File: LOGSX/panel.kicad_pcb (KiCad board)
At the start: 4 copper layers, 84 x 98 mm, 18 parts

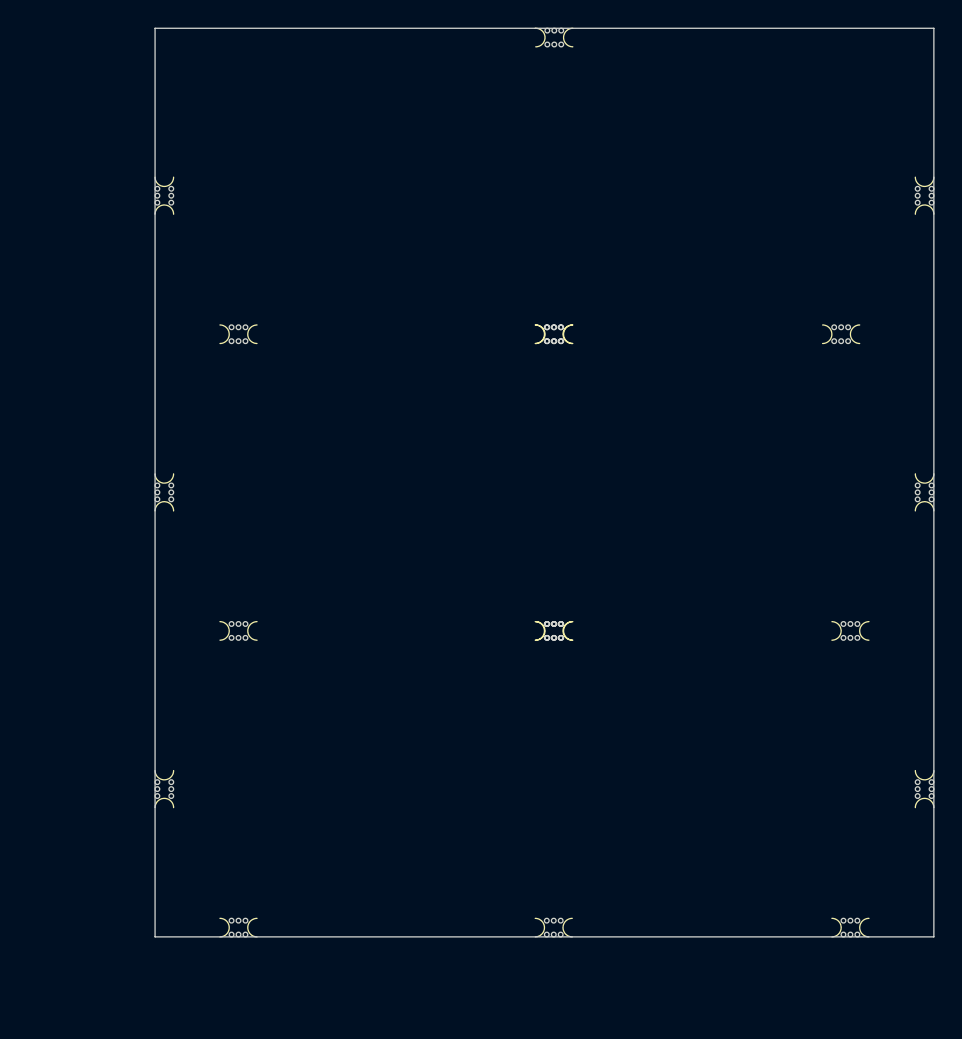
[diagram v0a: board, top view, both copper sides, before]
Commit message: Add files via upload
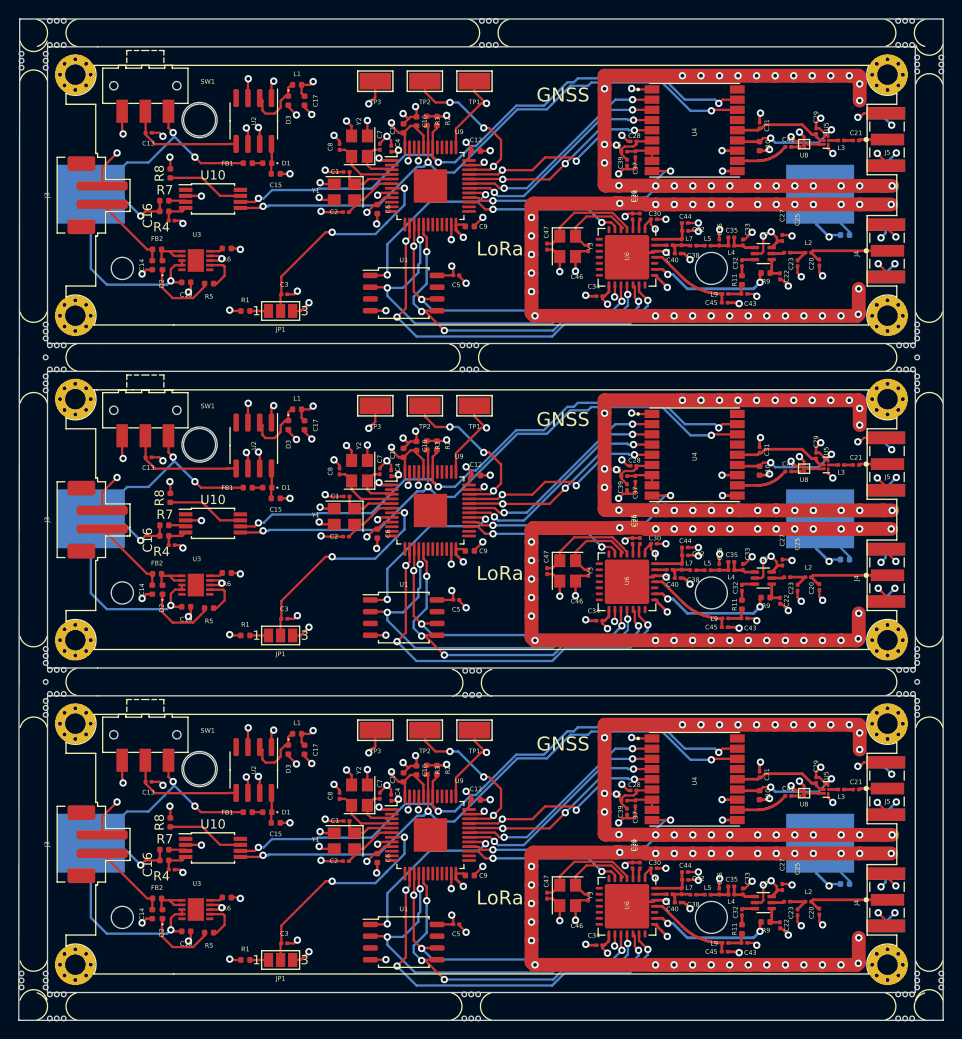
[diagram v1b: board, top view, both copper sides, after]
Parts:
- removed mouse-bite-2mm-slot (x18): VAL**, ASSETS:mouse-bite-2mm-slot
- added C1: 2.2pF, Capacitor_SMD:C_0201_0603Metric, F.Cu at (162.7, 138.5)
- added C1: 2.2pF, Capacitor_SMD:C_0201_0603Metric, F.Cu at (162.7, 103.5)
- added C1: 2.2pF, Capacitor_SMD:C_0201_0603Metric, F.Cu at (162.7, 68.5)
- added C10: 2.2pF, Capacitor_SMD:C_0402_1005Metric, F.Cu at (170.2, 133.0)
- added C10: 2.2pF, Capacitor_SMD:C_0402_1005Metric, F.Cu at (170.2, 98.0)
- added C10: 2.2pF, Capacitor_SMD:C_0402_1005Metric, F.Cu at (170.2, 63.0)
- added C11: 2.2pF, Capacitor_SMD:C_0402_1005Metric, F.Cu at (168.8, 133.8)
- added C11: 2.2pF, Capacitor_SMD:C_0402_1005Metric, F.Cu at (168.8, 98.8)
- added C11: 2.2pF, Capacitor_SMD:C_0402_1005Metric, F.Cu at (168.8, 63.8)
- added C12: 2.2pF, Capacitor_SMD:C_0402_1005Metric, F.Cu at (176.6, 136.2)
- added C12: 2.2pF, Capacitor_SMD:C_0402_1005Metric, F.Cu at (176.6, 101.2)
- added C12: 2.2pF, Capacitor_SMD:C_0402_1005Metric, F.Cu at (176.6, 66.2)
- added C13: 1nF, Capacitor_SMD:C_0201_0603Metric, F.Cu at (141.3, 134.3)
- added C13: 1nF, Capacitor_SMD:C_0201_0603Metric, F.Cu at (141.3, 99.3)
- added C13: 1nF, Capacitor_SMD:C_0201_0603Metric, F.Cu at (141.3, 64.3)
- added C14: 22pF, Capacitor_SMD:C_0402_1005Metric, F.Cu at (141.7, 148.6)
- added C14: 22pF, Capacitor_SMD:C_0402_1005Metric, F.Cu at (141.7, 113.5)
- added C14: 22pF, Capacitor_SMD:C_0402_1005Metric, F.Cu at (141.7, 78.5)
- added C15: 1uF, Capacitor_SMD:C_0402_1005Metric, F.Cu at (155.0, 138.7)
- added C15: 1uF, Capacitor_SMD:C_0402_1005Metric, F.Cu at (155.0, 103.7)
- added C15: 1uF, Capacitor_SMD:C_0402_1005Metric, F.Cu at (155.0, 68.7)
- added C16: 1nF, Capacitor_SMD:C_0201_0603Metric, F.Cu at (143.8, 143.8)
- added C16: 1nF, Capacitor_SMD:C_0201_0603Metric, F.Cu at (143.8, 108.8)
- added C16: 1nF, Capacitor_SMD:C_0201_0603Metric, F.Cu at (143.8, 73.8)
- added C17: 330uF, Capacitor_SMD:C_0402_1005Metric, F.Cu at (158.1, 130.8)
- added C17: 330uF, Capacitor_SMD:C_0402_1005Metric, F.Cu at (158.1, 95.8)
- added C17: 330uF, Capacitor_SMD:C_0402_1005Metric, F.Cu at (158.1, 60.8)
- added C19: 22pF, Capacitor_SMD:C_0402_1005Metric, F.Cu at (145.4, 150.4)
- added C19: 22pF, Capacitor_SMD:C_0402_1005Metric, F.Cu at (145.4, 115.4)
- added C19: 22pF, Capacitor_SMD:C_0402_1005Metric, F.Cu at (145.4, 80.4)
- added C2: 2.2pF, Capacitor_SMD:C_0201_0603Metric, F.Cu at (162.6, 142.8)
- added C2: 2.2pF, Capacitor_SMD:C_0201_0603Metric, F.Cu at (162.6, 107.8)
- added C2: 2.2pF, Capacitor_SMD:C_0201_0603Metric, F.Cu at (162.6, 72.8)
- added C20: X, Capacitor_SMD:C_0201_0603Metric, F.Cu at (213.7, 148.3)
- added C20: X, Capacitor_SMD:C_0201_0603Metric, F.Cu at (213.7, 113.3)
- added C20: X, Capacitor_SMD:C_0201_0603Metric, F.Cu at (213.7, 78.3)
- added C21: 120pF, Capacitor_SMD:C_0201_0603Metric, F.Cu at (217.6, 135.1)
- added C21: 120pF, Capacitor_SMD:C_0201_0603Metric, F.Cu at (217.6, 100.1)
- added C21: 120pF, Capacitor_SMD:C_0201_0603Metric, F.Cu at (217.6, 65.1)
- added C22: 1nF, Capacitor_SMD:C_0201_0603Metric, F.Cu at (209.4, 149.8)
- added C22: 1nF, Capacitor_SMD:C_0201_0603Metric, F.Cu at (209.4, 114.8)
- added C22: 1nF, Capacitor_SMD:C_0201_0603Metric, F.Cu at (209.4, 79.8)
- added C23: X, Capacitor_SMD:C_0201_0603Metric, F.Cu at (211.3, 148.3)
- added C23: X, Capacitor_SMD:C_0201_0603Metric, F.Cu at (211.3, 113.3)
- added C23: X, Capacitor_SMD:C_0201_0603Metric, F.Cu at (211.3, 78.3)
- added C24: 100nF, Capacitor_SMD:C_0201_0603Metric, F.Cu at (194.3, 143.3)
- added C24: 100nF, Capacitor_SMD:C_0201_0603Metric, F.Cu at (194.3, 108.3)
- added C24: 100nF, Capacitor_SMD:C_0201_0603Metric, F.Cu at (194.3, 73.3)
- added C25: X, Capacitor_SMD:C_0201_0603Metric, F.Cu at (210.2, 147.2)
- added C25: X, Capacitor_SMD:C_0201_0603Metric, F.Cu at (210.2, 112.2)
- added C25: X, Capacitor_SMD:C_0201_0603Metric, F.Cu at (210.2, 77.2)
- added C26: 100nF, Capacitor_SMD:C_0201_0603Metric, F.Cu at (193.5, 143.3)
- added C26: 100nF, Capacitor_SMD:C_0201_0603Metric, F.Cu at (193.5, 108.3)
- added C26: 100nF, Capacitor_SMD:C_0201_0603Metric, F.Cu at (193.5, 73.3)
- added C27: 1nF, Capacitor_SMD:C_0201_0603Metric, F.Cu at (209.7, 145.6)
- added C27: 1nF, Capacitor_SMD:C_0201_0603Metric, F.Cu at (209.7, 110.6)
- added C27: 1nF, Capacitor_SMD:C_0201_0603Metric, F.Cu at (209.7, 75.6)
- added C28: 56pF, Capacitor_SMD:C_0201_0603Metric, F.Cu at (193.6, 135.2)
- added C28: 56pF, Capacitor_SMD:C_0201_0603Metric, F.Cu at (193.6, 100.2)
- added C28: 56pF, Capacitor_SMD:C_0201_0603Metric, F.Cu at (193.6, 65.2)
- added C29: 1nF, Capacitor_SMD:C_0201_0603Metric, F.Cu at (213.3, 134.1)
- added C29: 1nF, Capacitor_SMD:C_0201_0603Metric, F.Cu at (213.3, 99.1)
- added C29: 1nF, Capacitor_SMD:C_0201_0603Metric, F.Cu at (213.3, 64.1)
- added C3: 2.2pF, Capacitor_SMD:C_0201_0603Metric, F.Cu at (155.9, 151.7)
- added C3: 2.2pF, Capacitor_SMD:C_0201_0603Metric, F.Cu at (155.9, 116.7)
- added C3: 2.2pF, Capacitor_SMD:C_0201_0603Metric, F.Cu at (155.9, 81.7)
- added C30: 100nF, Capacitor_SMD:C_0201_0603Metric, F.Cu at (195.8, 143.6)
- added C30: 100nF, Capacitor_SMD:C_0201_0603Metric, F.Cu at (195.8, 108.6)
- added C30: 100nF, Capacitor_SMD:C_0201_0603Metric, F.Cu at (195.8, 73.6)
- added C31: 56pF, Capacitor_SMD:C_0201_0603Metric, F.Cu at (207.2, 133.5)
- added C31: 56pF, Capacitor_SMD:C_0201_0603Metric, F.Cu at (207.2, 98.5)
- added C31: 56pF, Capacitor_SMD:C_0201_0603Metric, F.Cu at (207.2, 63.5)
- added C32: 120pF, Capacitor_SMD:C_0201_0603Metric, F.Cu at (205.3, 148.3)
- added C32: 120pF, Capacitor_SMD:C_0201_0603Metric, F.Cu at (205.3, 113.3)
- added C32: 120pF, Capacitor_SMD:C_0201_0603Metric, F.Cu at (205.3, 78.3)
- added C33: X, Capacitor_SMD:C_0201_0603Metric, F.Cu at (205.4, 146.1)
- added C33: X, Capacitor_SMD:C_0201_0603Metric, F.Cu at (205.4, 111.1)
- added C33: X, Capacitor_SMD:C_0201_0603Metric, F.Cu at (205.4, 76.1)
- added C34: 100nF, Capacitor_SMD:C_0201_0603Metric, F.Cu at (189.9, 151.9)
- added C34: 100nF, Capacitor_SMD:C_0201_0603Metric, F.Cu at (189.9, 116.9)
- added C34: 100nF, Capacitor_SMD:C_0201_0603Metric, F.Cu at (189.9, 81.9)
- added C35: X, Capacitor_SMD:C_0201_0603Metric, F.Cu at (204.2, 145.6)
- added C35: X, Capacitor_SMD:C_0201_0603Metric, F.Cu at (204.2, 110.5)
- added C35: X, Capacitor_SMD:C_0201_0603Metric, F.Cu at (204.2, 75.5)
- added C36: X, Capacitor_SMD:C_0201_0603Metric, F.Cu at (202.8, 146.1)
- added C36: X, Capacitor_SMD:C_0201_0603Metric, F.Cu at (202.8, 111.1)
- added C36: X, Capacitor_SMD:C_0201_0603Metric, F.Cu at (202.8, 76.1)
- added C37: 56pF, Capacitor_SMD:C_0201_0603Metric, F.Cu at (193.8, 136.6)
- added C37: 56pF, Capacitor_SMD:C_0201_0603Metric, F.Cu at (193.8, 101.6)
- added C37: 56pF, Capacitor_SMD:C_0201_0603Metric, F.Cu at (193.8, 66.6)
- added C38: X, Capacitor_SMD:C_0201_0603Metric, F.Cu at (200.1, 146.4)
- added C38: X, Capacitor_SMD:C_0201_0603Metric, F.Cu at (200.1, 111.5)
- added C38: X, Capacitor_SMD:C_0201_0603Metric, F.Cu at (200.1, 76.5)
- added C39: 56pF, Capacitor_SMD:C_0201_0603Metric, F.Cu at (192.9, 137.5)
- added C39: 56pF, Capacitor_SMD:C_0201_0603Metric, F.Cu at (192.9, 102.5)
- added C39: 56pF, Capacitor_SMD:C_0201_0603Metric, F.Cu at (192.9, 67.5)
- added C4: 2.2pF, Capacitor_SMD:C_0201_0603Metric, F.Cu at (167.5, 136.0)
- added C4: 2.2pF, Capacitor_SMD:C_0201_0603Metric, F.Cu at (167.5, 101.0)
- added C4: 2.2pF, Capacitor_SMD:C_0201_0603Metric, F.Cu at (167.5, 66.0)
- added C40: X, Capacitor_SMD:C_0201_0603Metric, F.Cu at (198.4, 147.3)
- added C40: X, Capacitor_SMD:C_0201_0603Metric, F.Cu at (198.4, 112.3)
- added C40: X, Capacitor_SMD:C_0201_0603Metric, F.Cu at (198.4, 77.3)
- added C41: 120pF, Capacitor_SMD:C_0201_0603Metric, F.Cu at (210.3, 135.8)
- added C41: 120pF, Capacitor_SMD:C_0201_0603Metric, F.Cu at (210.3, 100.8)
- added C41: 120pF, Capacitor_SMD:C_0201_0603Metric, F.Cu at (210.3, 65.8)
- added C42: X, Capacitor_SMD:C_0201_0603Metric, F.Cu at (199.2, 144.8)
- added C42: X, Capacitor_SMD:C_0201_0603Metric, F.Cu at (199.2, 109.8)
- added C42: X, Capacitor_SMD:C_0201_0603Metric, F.Cu at (199.2, 74.8)
- added C43: X, Capacitor_SMD:C_0201_0603Metric, F.Cu at (205.6, 151.7)
- added C43: X, Capacitor_SMD:C_0201_0603Metric, F.Cu at (205.6, 116.7)
- added C43: X, Capacitor_SMD:C_0201_0603Metric, F.Cu at (205.6, 81.7)
- added C44: X, Capacitor_SMD:C_0201_0603Metric, F.Cu at (199.2, 144.0)
- added C44: X, Capacitor_SMD:C_0201_0603Metric, F.Cu at (199.2, 109.0)
- added C44: X, Capacitor_SMD:C_0201_0603Metric, F.Cu at (199.2, 74.0)
- added C45: X, Capacitor_SMD:C_0201_0603Metric, F.Cu at (203.4, 152.6)
- added C45: X, Capacitor_SMD:C_0201_0603Metric, F.Cu at (203.4, 117.6)
- added C45: X, Capacitor_SMD:C_0201_0603Metric, F.Cu at (203.4, 82.6)
- added C46: 2.2pF, Capacitor_SMD:C_0201_0603Metric, F.Cu at (188.7, 146.7)
- added C46: 2.2pF, Capacitor_SMD:C_0201_0603Metric, F.Cu at (188.7, 111.7)
- added C46: 2.2pF, Capacitor_SMD:C_0201_0603Metric, F.Cu at (188.7, 76.7)
- added C47: 2.2pF, Capacitor_SMD:C_0201_0603Metric, F.Cu at (184.3, 146.6)
- added C47: 2.2pF, Capacitor_SMD:C_0201_0603Metric, F.Cu at (184.3, 111.5)
- added C47: 2.2pF, Capacitor_SMD:C_0201_0603Metric, F.Cu at (184.3, 76.5)
- added C5: 2.2pF, Capacitor_SMD:C_0201_0603Metric, F.Cu at (174.5, 149.6)
- added C5: 2.2pF, Capacitor_SMD:C_0201_0603Metric, F.Cu at (174.5, 114.6)
- added C5: 2.2pF, Capacitor_SMD:C_0201_0603Metric, F.Cu at (174.5, 79.6)
- added C6: 1uF, Capacitor_SMD:C_0402_1005Metric, F.Cu at (166.0, 142.5)
- added C6: 1uF, Capacitor_SMD:C_0402_1005Metric, F.Cu at (166.0, 107.5)
- added C6: 1uF, Capacitor_SMD:C_0402_1005Metric, F.Cu at (166.0, 72.5)
- added C7: 1pF, Capacitor_SMD:C_0201_0603Metric, F.Cu at (166.2, 135.8)
- added C7: 1pF, Capacitor_SMD:C_0201_0603Metric, F.Cu at (166.2, 100.8)
- added C7: 1pF, Capacitor_SMD:C_0201_0603Metric, F.Cu at (166.2, 65.8)
- added C8: 1pF, Capacitor_SMD:C_0201_0603Metric, F.Cu at (161.9, 135.8)
- added C8: 1pF, Capacitor_SMD:C_0201_0603Metric, F.Cu at (161.9, 100.8)
- added C8: 1pF, Capacitor_SMD:C_0201_0603Metric, F.Cu at (161.9, 65.8)
- added C9: 2.2pF, Capacitor_SMD:C_0402_1005Metric, F.Cu at (175.9, 144.4)
- added C9: 2.2pF, Capacitor_SMD:C_0402_1005Metric, F.Cu at (175.9, 109.4)
- added C9: 2.2pF, Capacitor_SMD:C_0402_1005Metric, F.Cu at (175.9, 74.4)
- added D1: D_Small, Diode_SMD:D_0402_1005Metric, F.Cu at (154.1, 137.6)
- added D1: D_Small, Diode_SMD:D_0402_1005Metric, F.Cu at (154.1, 102.5)
- added D1: D_Small, Diode_SMD:D_0402_1005Metric, F.Cu at (154.1, 67.5)
- added D2: LED, LED_SMD:LED_0402_1005Metric, F.Cu at (142.8, 148.6)
- added D2: LED, LED_SMD:LED_0402_1005Metric, F.Cu at (142.8, 113.5)
- added D2: LED, LED_SMD:LED_0402_1005Metric, F.Cu at (142.8, 78.5)
- added D3: 1N5822, Diode_SMD:D_0402_1005Metric, F.Cu at (156.4, 130.8)
- added D3: 1N5822, Diode_SMD:D_0402_1005Metric, F.Cu at (156.4, 95.8)
- added D3: 1N5822, Diode_SMD:D_0402_1005Metric, F.Cu at (156.4, 60.8)
- added FB1: 100MHz, Inductor_SMD:L_0402_1005Metric, F.Cu at (152.0, 137.6)
- added FB1: 100MHz, Inductor_SMD:L_0402_1005Metric, F.Cu at (152.0, 102.5)
- added FB1: 100MHz, Inductor_SMD:L_0402_1005Metric, F.Cu at (152.0, 67.5)
- added FB2: 100MHz, Inductor_SMD:L_0402_1005Metric, F.Cu at (142.2, 146.8)
- added FB2: 100MHz, Inductor_SMD:L_0402_1005Metric, F.Cu at (142.2, 111.8)
- added FB2: 100MHz, Inductor_SMD:L_0402_1005Metric, F.Cu at (142.2, 76.8)
- added J2: BATTERY CONN, Battery:BatteryHolder_Keystone_1042_1x18650, B.Cu at (174.4, 140.9)
- added J2: BATTERY CONN, Battery:BatteryHolder_Keystone_1042_1x18650, B.Cu at (174.4, 105.9)
- added J2: BATTERY CONN, Battery:BatteryHolder_Keystone_1042_1x18650, B.Cu at (174.4, 70.9)
- added J3: POWER IN, Connector_JST:JST_PH_B2B-PH-SM4-TB_1x02-1MP_P2.00mm_Vertical, F.Cu at (135.8, 141.0)
- added J3: POWER IN, Connector_JST:JST_PH_B2B-PH-SM4-TB_1x02-1MP_P2.00mm_Vertical, F.Cu at (135.8, 106.0)
- added J3: POWER IN, Connector_JST:JST_PH_B2B-PH-SM4-TB_1x02-1MP_P2.00mm_Vertical, F.Cu at (135.8, 71.0)
- added J4: SMA_Edge, ASSETS:SMA-J-P-H-ST-EM1, F.Cu at (221.0, 147.0)
- added J4: SMA_Edge, ASSETS:SMA-J-P-H-ST-EM1, F.Cu at (221.0, 112.0)
- added J4: SMA_Edge, ASSETS:SMA-J-P-H-ST-EM1, F.Cu at (221.0, 77.0)
- added J5: SMA_Edge, ASSETS:SMA-J-P-H-ST-EM1, F.Cu at (221.0, 135.0)
- added J5: SMA_Edge, ASSETS:SMA-J-P-H-ST-EM1, F.Cu at (221.0, 100.0)
- added J5: SMA_Edge, ASSETS:SMA-J-P-H-ST-EM1, F.Cu at (221.0, 65.0)
- added JP1: SolderJumper_3_Open, Jumper:SolderJumper-3_P1.3mm_Open_Pad1.0x1.5mm_NumberLabels, F.Cu at (155.5, 153.5)
- added JP1: SolderJumper_3_Open, Jumper:SolderJumper-3_P1.3mm_Open_Pad1.0x1.5mm_NumberLabels, F.Cu at (155.5, 118.5)
- added JP1: SolderJumper_3_Open, Jumper:SolderJumper-3_P1.3mm_Open_Pad1.0x1.5mm_NumberLabels, F.Cu at (155.5, 83.5)
- added L1: 330uH, Inductor_SMD:L_0402_1005Metric, F.Cu at (157.3, 129.1)
- added L1: 330uH, Inductor_SMD:L_0402_1005Metric, F.Cu at (157.3, 94.1)
- added L1: 330uH, Inductor_SMD:L_0402_1005Metric, F.Cu at (157.3, 59.1)
- added L2: X, Inductor_SMD:L_0201_0603Metric, F.Cu at (212.4, 147.2)
- added L2: X, Inductor_SMD:L_0201_0603Metric, F.Cu at (212.4, 112.2)
- added L2: X, Inductor_SMD:L_0201_0603Metric, F.Cu at (212.4, 77.2)
- added L3: 5nF, Inductor_SMD:L_0201_0603Metric, F.Cu at (216.0, 135.1)
- added L3: 5nF, Inductor_SMD:L_0201_0603Metric, F.Cu at (216.0, 100.1)
- added L3: 5nF, Inductor_SMD:L_0201_0603Metric, F.Cu at (216.0, 65.1)
- added L4: X, Inductor_SMD:L_0201_0603Metric, F.Cu at (204.2, 146.4)
- added L4: X, Inductor_SMD:L_0201_0603Metric, F.Cu at (204.2, 111.5)
- added L4: X, Inductor_SMD:L_0201_0603Metric, F.Cu at (204.2, 76.5)
- added L5: X, Inductor_SMD:L_0201_0603Metric, F.Cu at (201.6, 146.4)
- added L5: X, Inductor_SMD:L_0201_0603Metric, F.Cu at (201.6, 111.5)
- added L5: X, Inductor_SMD:L_0201_0603Metric, F.Cu at (201.6, 76.5)
- added L6: 27nH, Inductor_SMD:L_0201_0603Metric, F.Cu at (192.6, 136.3)
- added L6: 27nH, Inductor_SMD:L_0201_0603Metric, F.Cu at (192.6, 101.3)
- added L6: 27nH, Inductor_SMD:L_0201_0603Metric, F.Cu at (192.6, 66.3)
- added L7: X, Inductor_SMD:L_0201_0603Metric, F.Cu at (198.8, 146.1)
- added L7: X, Inductor_SMD:L_0201_0603Metric, F.Cu at (198.8, 111.1)
- added L7: X, Inductor_SMD:L_0201_0603Metric, F.Cu at (198.8, 76.1)
- added L8: X, Inductor_SMD:L_0201_0603Metric, F.Cu at (197.5, 146.4)
- added L8: X, Inductor_SMD:L_0201_0603Metric, F.Cu at (197.5, 111.4)
- added L8: X, Inductor_SMD:L_0201_0603Metric, F.Cu at (197.5, 76.4)
- added L9: X, Inductor_SMD:L_0201_0603Metric, F.Cu at (203.5, 151.7)
- added L9: X, Inductor_SMD:L_0201_0603Metric, F.Cu at (203.5, 116.7)
- added L9: X, Inductor_SMD:L_0201_0603Metric, F.Cu at (203.5, 81.7)
- added R1: 1K7, Resistor_SMD:R_0402_1005Metric, F.Cu at (151.7, 153.5)
- added R1: 1K7, Resistor_SMD:R_0402_1005Metric, F.Cu at (151.7, 118.5)
- added R1: 1K7, Resistor_SMD:R_0402_1005Metric, F.Cu at (151.7, 83.5)
- added R10: 10K, Resistor_SMD:R_0402_1005Metric, F.Cu at (207.2, 135.7)
- added R10: 10K, Resistor_SMD:R_0402_1005Metric, F.Cu at (207.2, 100.7)
- added R10: 10K, Resistor_SMD:R_0402_1005Metric, F.Cu at (207.2, 65.7)
- added R11: 0, Resistor_SMD:R_0402_1005Metric, F.Cu at (205.3, 150.2)
- added R11: 0, Resistor_SMD:R_0402_1005Metric, F.Cu at (205.3, 115.2)
- added R11: 0, Resistor_SMD:R_0402_1005Metric, F.Cu at (205.3, 80.2)
- added R2: 4.7K, Resistor_SMD:R_0402_1005Metric, F.Cu at (172.4, 133.0)
- added R2: 4.7K, Resistor_SMD:R_0402_1005Metric, F.Cu at (172.4, 98.0)
- added R2: 4.7K, Resistor_SMD:R_0402_1005Metric, F.Cu at (172.4, 63.0)
- added R3: 4.7K, Resistor_SMD:R_0402_1005Metric, F.Cu at (171.3, 133.0)
- added R3: 4.7K, Resistor_SMD:R_0402_1005Metric, F.Cu at (171.3, 98.0)
- added R3: 4.7K, Resistor_SMD:R_0402_1005Metric, F.Cu at (171.3, 63.0)
- added R4: R_Small, Resistor_SMD:R_0402_1005Metric, B.Cu at (216.4, 145.3)
- added R4: R_Small, Resistor_SMD:R_0402_1005Metric, B.Cu at (216.4, 110.3)
- added R4: 500, Resistor_SMD:R_0402_1005Metric, F.Cu at (143.0, 142.8)
- added R4: 500, Resistor_SMD:R_0402_1005Metric, F.Cu at (143.0, 107.8)
- added R4: 500, Resistor_SMD:R_0402_1005Metric, F.Cu at (143.0, 72.8)
- added R4: R_Small, Resistor_SMD:R_0402_1005Metric, B.Cu at (216.4, 75.3)
- added R5: 1K, Resistor_SMD:R_0402_1005Metric, F.Cu at (147.8, 150.5)
- added R5: 1K, Resistor_SMD:R_0402_1005Metric, F.Cu at (147.8, 115.5)
- added R5: 1K, Resistor_SMD:R_0402_1005Metric, F.Cu at (147.8, 80.5)
- added R6: 1K, Resistor_SMD:R_0402_1005Metric, F.Cu at (149.7, 146.8)
- added R6: 1K, Resistor_SMD:R_0402_1005Metric, F.Cu at (149.7, 111.8)
- added R6: 1K, Resistor_SMD:R_0402_1005Metric, F.Cu at (149.7, 76.8)
- added R7: 1K, Resistor_SMD:R_0402_1005Metric, F.Cu at (143.0, 141.6)
- added R7: 1K, Resistor_SMD:R_0402_1005Metric, F.Cu at (143.0, 106.6)
- added R7: 1K, Resistor_SMD:R_0402_1005Metric, F.Cu at (143.0, 71.6)
- added R8: 1K, Resistor_SMD:R_0402_1005Metric, F.Cu at (143.7, 138.7)
- added R8: 1K, Resistor_SMD:R_0402_1005Metric, F.Cu at (143.7, 103.7)
- added R8: 1K, Resistor_SMD:R_0402_1005Metric, F.Cu at (143.7, 68.7)
- added R9: 1K, Resistor_SMD:R_0402_1005Metric, F.Cu at (207.8, 149.4)
- added R9: 1K, Resistor_SMD:R_0402_1005Metric, F.Cu at (207.8, 114.4)
- added R9: 1K, Resistor_SMD:R_0402_1005Metric, F.Cu at (207.8, 79.4)
- added REF**: MountingHole_2.2mm_M2_Pad_Via, MountingHole:MountingHole_2.2mm_M2_Pad_Via, F.Cu at (221.0, 154.0)
- added REF**: MountingHole_2.2mm_M2_Pad_Via, MountingHole:MountingHole_2.2mm_M2_Pad_Via, F.Cu at (221.0, 58.0)
- added REF**: MountingHole_2.2mm_M2_Pad_Via, MountingHole:MountingHole_2.2mm_M2_Pad_Via, F.Cu at (133.4, 84.0)
- added REF**: MountingHole_2.2mm_M2_Pad_Via, MountingHole:MountingHole_2.2mm_M2_Pad_Via, F.Cu at (133.4, 58.0)
- added REF**: MountingHole_2.2mm_M2_Pad_Via, MountingHole:MountingHole_2.2mm_M2_Pad_Via, F.Cu at (221.0, 119.0)
- added REF**: MountingHole_2.2mm_M2_Pad_Via, MountingHole:MountingHole_2.2mm_M2_Pad_Via, F.Cu at (221.0, 128.0)
- added REF**: MountingHole_2.2mm_M2_Pad_Via, MountingHole:MountingHole_2.2mm_M2_Pad_Via, F.Cu at (221.0, 93.0)
- added REF**: MountingHole_2.2mm_M2_Pad_Via, MountingHole:MountingHole_2.2mm_M2_Pad_Via, F.Cu at (133.4, 128.0)
- added REF**: MountingHole_2.2mm_M2_Pad_Via, MountingHole:MountingHole_2.2mm_M2_Pad_Via, F.Cu at (133.4, 93.0)
- added REF**: MountingHole_2.2mm_M2_Pad_Via, MountingHole:MountingHole_2.2mm_M2_Pad_Via, F.Cu at (133.4, 154.0)
- added REF**: MountingHole_2.2mm_M2_Pad_Via, MountingHole:MountingHole_2.2mm_M2_Pad_Via, F.Cu at (133.4, 119.0)
- added REF**: MountingHole_2.2mm_M2_Pad_Via, MountingHole:MountingHole_2.2mm_M2_Pad_Via, F.Cu at (221.0, 84.0)
- added SW1: SW_SPDT, Button_Switch_SMD:SW_SPDT_CK-JS102011SAQN, F.Cu at (140.9, 129.2)
- added SW1: SW_SPDT, Button_Switch_SMD:SW_SPDT_CK-JS102011SAQN, F.Cu at (140.9, 94.2)
- added SW1: SW_SPDT, Button_Switch_SMD:SW_SPDT_CK-JS102011SAQN, F.Cu at (140.9, 59.2)
- added TP1: TestPoint, TestPoint:TestPoint_Keystone_5015_Micro-Minature, F.Cu at (176.4, 128.7)
- added TP1: TestPoint, TestPoint:TestPoint_Keystone_5015_Micro-Minature, F.Cu at (176.4, 93.7)
- added TP1: TestPoint, TestPoint:TestPoint_Keystone_5015_Micro-Minature, F.Cu at (176.4, 58.7)
- added TP2: TestPoint, TestPoint:TestPoint_Keystone_5015_Micro-Minature, F.Cu at (171.1, 128.7)
- added TP2: TestPoint, TestPoint:TestPoint_Keystone_5015_Micro-Minature, F.Cu at (171.1, 93.7)
- added TP2: TestPoint, TestPoint:TestPoint_Keystone_5015_Micro-Minature, F.Cu at (171.1, 58.7)
- added TP3: TestPoint, TestPoint:TestPoint_Keystone_5015_Micro-Minature, F.Cu at (165.8, 128.7)
- added TP3: TestPoint, TestPoint:TestPoint_Keystone_5015_Micro-Minature, F.Cu at (165.8, 93.7)
- added TP3: TestPoint, TestPoint:TestPoint_Keystone_5015_Micro-Minature, F.Cu at (165.8, 58.7)
- added U1: W25Q32JVSS, Package_SO:SOIC-8_5.23x5.23mm_P1.27mm, F.Cu at (168.8, 151.6)
- added U1: W25Q32JVSS, Package_SO:SOIC-8_5.23x5.23mm_P1.27mm, F.Cu at (168.8, 116.6)
- added U1: W25Q32JVSS, Package_SO:SOIC-8_5.23x5.23mm_P1.27mm, F.Cu at (168.8, 81.6)
- added U10: DS2782, Package_SO:TSSOP-8_4.4x3mm_P0.65mm, F.Cu at (148.2, 141.4)
- added U10: DS2782, Package_SO:TSSOP-8_4.4x3mm_P0.65mm, F.Cu at (148.2, 106.4)
- added U10: DS2782, Package_SO:TSSOP-8_4.4x3mm_P0.65mm, F.Cu at (148.2, 71.4)
- added U2: LT1129-3.3_SO8, Package_SO:SOIC-8_3.9x4.9mm_P1.27mm, F.Cu at (152.7, 133.0)
- added U2: LT1129-3.3_SO8, Package_SO:SOIC-8_3.9x4.9mm_P1.27mm, F.Cu at (152.7, 98.0)
- added U2: LT1129-3.3_SO8, Package_SO:SOIC-8_3.9x4.9mm_P1.27mm, F.Cu at (152.7, 63.0)
- added U3: MCP73113_4, ASSETS:MCP73113, F.Cu at (146.4, 148.1)
- added U3: MCP73113_4, ASSETS:MCP73113, F.Cu at (146.4, 113.0)
- added U3: MCP73113_4, ASSETS:MCP73113, F.Cu at (146.4, 78.0)
- added U4: TESEO-LIV3F, ASSETS:TESEO-LIV3F, F.Cu at (200.2, 134.0)
- added U4: TESEO-LIV3F, ASSETS:TESEO-LIV3F, F.Cu at (200.2, 99.0)
- added U4: TESEO-LIV3F, ASSETS:TESEO-LIV3F, F.Cu at (200.2, 64.0)
- added U5: BGA725L6E6327FTSA1, ASSETS:BGA725L6E6327FTSA1, F.Cu at (214.4, 135.1)
- added U5: BGA725L6E6327FTSA1, ASSETS:BGA725L6E6327FTSA1, F.Cu at (214.4, 100.1)
- added U5: BGA725L6E6327FTSA1, ASSETS:BGA725L6E6327FTSA1, F.Cu at (214.4, 65.1)
- added U6: SX1273, Package_DFN_QFN:QFN-28-1EP_6x6mm_P0.65mm_EP4.8x4.8mm, F.Cu at (192.9, 147.7)
- added U6: SX1273, Package_DFN_QFN:QFN-28-1EP_6x6mm_P0.65mm_EP4.8x4.8mm, F.Cu at (192.9, 112.7)
- added U6: SX1273, Package_DFN_QFN:QFN-28-1EP_6x6mm_P0.65mm_EP4.8x4.8mm, F.Cu at (192.9, 77.7)
- added U7: PE4259, ASSETS:PE4259_sc70, F.Cu at (207.6, 147.3)
- added U7: PE4259, ASSETS:PE4259_sc70, F.Cu at (207.6, 112.3)
- added U7: PE4259, ASSETS:PE4259_sc70, F.Cu at (207.6, 77.3)
- added U8: B4327, ASSETS:B4327, F.Cu at (212.0, 135.5)
- added U8: B4327, ASSETS:B4327, F.Cu at (212.0, 100.5)
- added U8: B4327, ASSETS:B4327, F.Cu at (212.0, 65.5)
- added U9: STM32F103C8Tx, Package_QFP:LQFP-48-1EP_7x7mm_P0.5mm_EP3.6x3.6mm, F.Cu at (171.7, 140.0)
- added U9: STM32F103C8Tx, Package_QFP:LQFP-48-1EP_7x7mm_P0.5mm_EP3.6x3.6mm, F.Cu at (171.7, 105.0)
- added U9: STM32F103C8Tx, Package_QFP:LQFP-48-1EP_7x7mm_P0.5mm_EP3.6x3.6mm, F.Cu at (171.7, 70.0)
- added Y1: Crystal_GND23, Crystal:Crystal_SMD_Abracon_ABM8G-4Pin_3.2x2.5mm, F.Cu at (162.4, 140.7)
- added Y1: Crystal_GND23, Crystal:Crystal_SMD_Abracon_ABM8G-4Pin_3.2x2.5mm, F.Cu at (162.4, 105.7)
- added Y1: Crystal_GND23, Crystal:Crystal_SMD_Abracon_ABM8G-4Pin_3.2x2.5mm, F.Cu at (162.4, 70.7)
- added Y2: Crystal_GND23, Crystal:Crystal_SMD_Abracon_ABM8G-4Pin_3.2x2.5mm, F.Cu at (164.1, 135.7)
- added Y2: Crystal_GND23, Crystal:Crystal_SMD_Abracon_ABM8G-4Pin_3.2x2.5mm, F.Cu at (164.1, 100.7)
- added Y2: Crystal_GND23, Crystal:Crystal_SMD_Abracon_ABM8G-4Pin_3.2x2.5mm, F.Cu at (164.1, 65.7)
- added Y3: Crystal_GND23, Crystal:Crystal_SMD_Abracon_ABM8G-4Pin_3.2x2.5mm, F.Cu at (186.5, 146.5)
- added Y3: Crystal_GND23, Crystal:Crystal_SMD_Abracon_ABM8G-4Pin_3.2x2.5mm, F.Cu at (186.5, 111.5)
- added Y3: Crystal_GND23, Crystal:Crystal_SMD_Abracon_ABM8G-4Pin_3.2x2.5mm, F.Cu at (186.5, 76.5)
- added mouse-bite-3mm-slot: VAL**, Panelization:mouse-bite-3mm-slot, F.Cu at (176.1, 158.5)
- added mouse-bite-3mm-slot: VAL**, Panelization:mouse-bite-3mm-slot, F.Cu at (178.0, 53.5)
- added mouse-bite-3mm-slot: VAL**, Panelization:mouse-bite-3mm-slot, F.Cu at (222.9, 53.5)
- added mouse-bite-3mm-slot: VAL**, Panelization:mouse-bite-3mm-slot, F.Cu at (131.4, 53.5)
- added mouse-bite-3mm-slot: VAL**, Panelization:mouse-bite-3mm-slot, F.Cu at (225.5, 155.7)
- added mouse-bite-3mm-slot: VAL**, Panelization:mouse-bite-3mm-slot, F.Cu at (222.9, 158.5)
- added mouse-bite-3mm-slot: VAL**, Panelization:mouse-bite-3mm-slot, F.Cu at (225.5, 56.9)
- added mouse-bite-3mm-slot: VAL**, Panelization:mouse-bite-3mm-slot, F.Cu at (128.9, 56.5)
- added mouse-bite-3mm-slot: VAL**, Panelization:mouse-bite-3mm-slot, F.Cu at (128.9, 155.7)
- added mouse-bite-3mm-slot: VAL**, Panelization:mouse-bite-3mm-slot, F.Cu at (131.4, 158.5)
- added mouse-bite-3mm-slot: VAL**, Panelization:mouse-bite-3mm-slot, F.Cu at (176.2, 123.6)
- added mouse-bite-3mm-slot: VAL**, Panelization:mouse-bite-3mm-slot, F.Cu at (175.9, 88.5)
- added mouse-bite-3mm-slot-3way: VAL**, Panelization:mouse-bite-3mm-slot-3way, F.Cu at (225.5, 123.5)
- added mouse-bite-3mm-slot-3way: VAL**, Panelization:mouse-bite-3mm-slot-3way, F.Cu at (225.5, 88.5)
- added mouse-bite-3mm-slot-3way: VAL**, Panelization:mouse-bite-3mm-slot-3way, F.Cu at (128.9, 123.5)
- added mouse-bite-3mm-slot-3way: VAL**, Panelization:mouse-bite-3mm-slot-3way, F.Cu at (128.9, 88.5)
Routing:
- net GND: track 0.00 -> 1003.8 mm, vias 0 -> 420
- net SCL: track 0.00 -> 196.6 mm, vias 0 -> 9
- net SDA: track 0.00 -> 196.4 mm, vias 0 -> 9
- net BATTERY: track 0.00 -> 165.8 mm, vias 0 -> 12
- net +3V3: track 0.00 -> 131.9 mm, vias 0 -> 45
- net LoRa_NSS: track 0.00 -> 127.4 mm, vias 0 -> 9
- net MISO: track 0.00 -> 127.0 mm, vias 0 -> 9
- net MOSI: track 0.00 -> 120.2 mm, vias 0 -> 12
- net SCK: track 0.00 -> 103.4 mm, vias 0 -> 9
- net RX: track 0.00 -> 71.8 mm, vias 0 -> 6
- net TX: track 0.00 -> 71.7 mm, vias 0 -> 6
- net Net-(C3-Pad1): track 0.00 -> 70.7 mm, vias 0 -> 6
- net 1PPS: track 0.00 -> 67.5 mm, vias 0 -> 9
- net WAKE_UP: track 0.00 -> 66.9 mm, vias 0 -> 9
- net FLASH_NSS: track 0.00 -> 59.5 mm, vias 0 -> 6
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- added copper zone on PWR, net +3V3
- added copper zone on F.Cu, net GND
- added copper zone on GND, net GND
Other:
- board size 84 x 98 mm -> 99.7 x 108 mm
- net class Default: clearance 0.2 -> 0.12
- rule trace_clearance: 0.2 -> 0.12
- rule trace_min: 0.2 -> 0.12
- board text added: "CUT OUT"
- board text added: "GNSS"
- board text added: "LoRa"
